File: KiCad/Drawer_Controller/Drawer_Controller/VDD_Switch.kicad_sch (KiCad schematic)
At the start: 5 parts, among them Q7 AO3400A, Q8 AO3401A

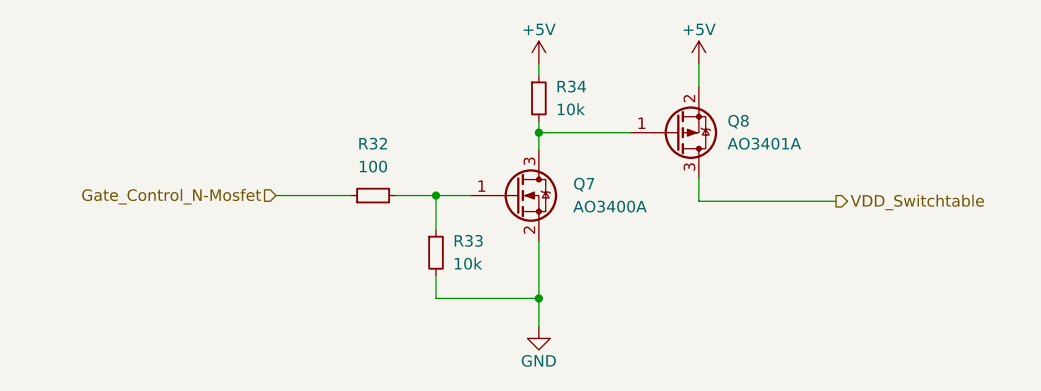
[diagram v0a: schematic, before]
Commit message: more progress, routing almost done
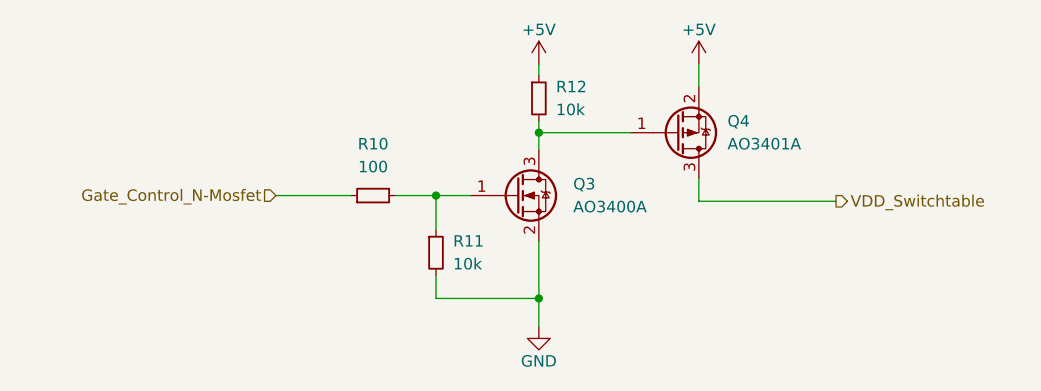
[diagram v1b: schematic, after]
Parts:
- renumbered Q7 to Q3, Q8 to Q4, R32 to R10, R33 to R11, R34 to R12
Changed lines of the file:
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@@
   (symbol (lib_id "power:+5V") (at 124.46 71.12 0)
     (in_bom yes) (on_board yes)
-    (property "Reference" "#PWR0159" (id 0) (at 124.46 74.93 0)
+    (property "Reference" "#PWR0115" (id 0) (at 124.46 74.93 0)
       (effects (font (size 1.27 1.27)) hide)
     )
@@
   (symbol (lib_id "Device:R_Small") (at 106.045 85.725 90)
     (in_bom yes) (on_board yes) (fields_autoplaced)
-    (property "Reference" "R32" (id 0) (at 106.045 80.01 90))
+    (property "Reference" "R10" (id 0) (at 106.045 80.01 90))
     (property "Value" "100" (id 1) (at 106.045 82.55 90))
     (property "Footprint" "Resistor_SMD:R_0805_2012Metric_Pad1.20x1.40mm_HandSolder" (id 2) (at 106.045 85.725 0)
@@
   (symbol (lib_id "Transistor_FET:AO3400A") (at 121.92 85.725 0)
     (in_bom yes) (on_board yes) (fields_autoplaced)
-    (property "Reference" "Q7" (id 0) (at 128.27 84.4549 0)
+    (property "Reference" "Q3" (id 0) (at 128.27 84.4549 0)
       (effects (font (size 1.27 1.27)) (justify left))
     )
@@
   (symbol (lib_id "power:+5V") (at 142.24 71.12 0)
     (in_bom yes) (on_board yes)
-    (property "Reference" "#PWR0161" (id 0) (at 142.24 74.93 0)
+    (property "Reference" "#PWR0121" (id 0) (at 142.24 74.93 0)
       (effects (font (size 1.27 1.27)) hide)
     )
@@
   (symbol (lib_id "Device:R_Small") (at 113.03 92.075 0)
     (in_bom yes) (on_board yes) (fields_autoplaced)
-    (property "Reference" "R33" (id 0) (at 114.935 90.8049 0)
+    (property "Reference" "R11" (id 0) (at 114.935 90.8049 0)
       (effects (font (size 1.27 1.27)) (justify left))
     )
@@
   (symbol (lib_id "Device:R_Small") (at 124.46 74.93 0)
     (in_bom yes) (on_board yes) (fields_autoplaced)
-    (property "Reference" "R34" (id 0) (at 126.365 73.6599 0)
+    (property "Reference" "R12" (id 0) (at 126.365 73.6599 0)
       (effects (font (size 1.27 1.27)) (justify left))
     )
@@
   (symbol (lib_id "power:GND") (at 124.46 100.33 0)
     (in_bom yes) (on_board yes)
-    (property "Reference" "#PWR0160" (id 0) (at 124.46 106.68 0)
+    (property "Reference" "#PWR0116" (id 0) (at 124.46 106.68 0)
       (effects (font (size 1.27 1.27)) hide)
     )
@@
   (symbol (lib_id "Transistor_FET:AO3401A") (at 139.7 78.74 0) (mirror x)
     (in_bom yes) (on_board yes) (fields_autoplaced)
-    (property "Reference" "Q8" (id 0) (at 145.415 77.4699 0)
+    (property "Reference" "Q4" (id 0) (at 145.415 77.4699 0)
       (effects (font (size 1.27 1.27)) (justify left))
     )

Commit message: Exported gerbers and small refinements
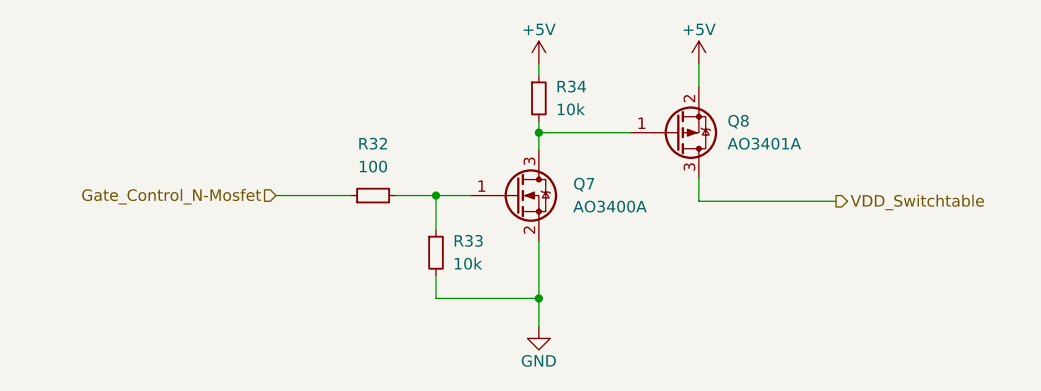
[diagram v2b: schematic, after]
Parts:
- renumbered Q3 to Q7, Q4 to Q8, R10 to R32, R11 to R33, R12 to R34
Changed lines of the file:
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@@
   (symbol (lib_id "power:+5V") (at 124.46 71.12 0)
     (in_bom yes) (on_board yes)
-    (property "Reference" "#PWR0115" (id 0) (at 124.46 74.93 0)
+    (property "Reference" "#PWR0159" (id 0) (at 124.46 74.93 0)
       (effects (font (size 1.27 1.27)) hide)
     )
@@
   (symbol (lib_id "Device:R_Small") (at 106.045 85.725 90)
     (in_bom yes) (on_board yes) (fields_autoplaced)
-    (property "Reference" "R10" (id 0) (at 106.045 80.01 90))
+    (property "Reference" "R32" (id 0) (at 106.045 80.01 90))
     (property "Value" "100" (id 1) (at 106.045 82.55 90))
     (property "Footprint" "Resistor_SMD:R_0805_2012Metric_Pad1.20x1.40mm_HandSolder" (id 2) (at 106.045 85.725 0)
@@
   (symbol (lib_id "Transistor_FET:AO3400A") (at 121.92 85.725 0)
     (in_bom yes) (on_board yes) (fields_autoplaced)
-    (property "Reference" "Q3" (id 0) (at 128.27 84.4549 0)
+    (property "Reference" "Q7" (id 0) (at 128.27 84.4549 0)
       (effects (font (size 1.27 1.27)) (justify left))
     )
@@
   (symbol (lib_id "power:+5V") (at 142.24 71.12 0)
     (in_bom yes) (on_board yes)
-    (property "Reference" "#PWR0121" (id 0) (at 142.24 74.93 0)
+    (property "Reference" "#PWR0161" (id 0) (at 142.24 74.93 0)
       (effects (font (size 1.27 1.27)) hide)
     )
@@
   (symbol (lib_id "Device:R_Small") (at 113.03 92.075 0)
     (in_bom yes) (on_board yes) (fields_autoplaced)
-    (property "Reference" "R11" (id 0) (at 114.935 90.8049 0)
+    (property "Reference" "R33" (id 0) (at 114.935 90.8049 0)
       (effects (font (size 1.27 1.27)) (justify left))
     )
@@
   (symbol (lib_id "Device:R_Small") (at 124.46 74.93 0)
     (in_bom yes) (on_board yes) (fields_autoplaced)
-    (property "Reference" "R12" (id 0) (at 126.365 73.6599 0)
+    (property "Reference" "R34" (id 0) (at 126.365 73.6599 0)
       (effects (font (size 1.27 1.27)) (justify left))
     )
@@
   (symbol (lib_id "power:GND") (at 124.46 100.33 0)
     (in_bom yes) (on_board yes)
-    (property "Reference" "#PWR0116" (id 0) (at 124.46 106.68 0)
+    (property "Reference" "#PWR0160" (id 0) (at 124.46 106.68 0)
       (effects (font (size 1.27 1.27)) hide)
     )
@@
   (symbol (lib_id "Transistor_FET:AO3401A") (at 139.7 78.74 0) (mirror x)
     (in_bom yes) (on_board yes) (fields_autoplaced)
-    (property "Reference" "Q4" (id 0) (at 145.415 77.4699 0)
+    (property "Reference" "Q8" (id 0) (at 145.415 77.4699 0)
       (effects (font (size 1.27 1.27)) (justify left))
     )
